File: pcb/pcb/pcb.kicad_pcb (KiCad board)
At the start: 2 copper layers, 66 x 44.5 mm, 20 parts, among them J1 UART, J2 Barrel_Jack, J3 Stepper, SW1 RESET, SW2 FLASH, U1 ESP32-WROOM-32, U2 TSR_1-2433

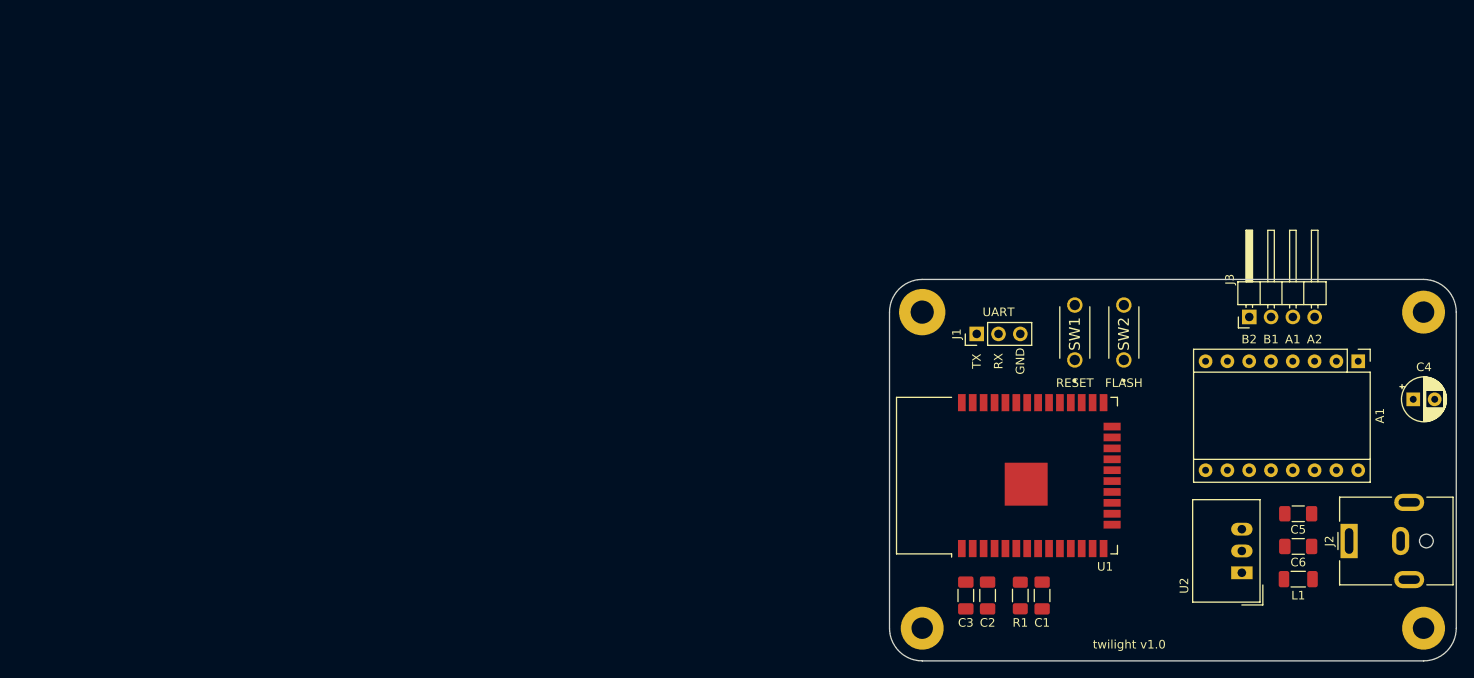
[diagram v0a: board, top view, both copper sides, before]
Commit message: route traces
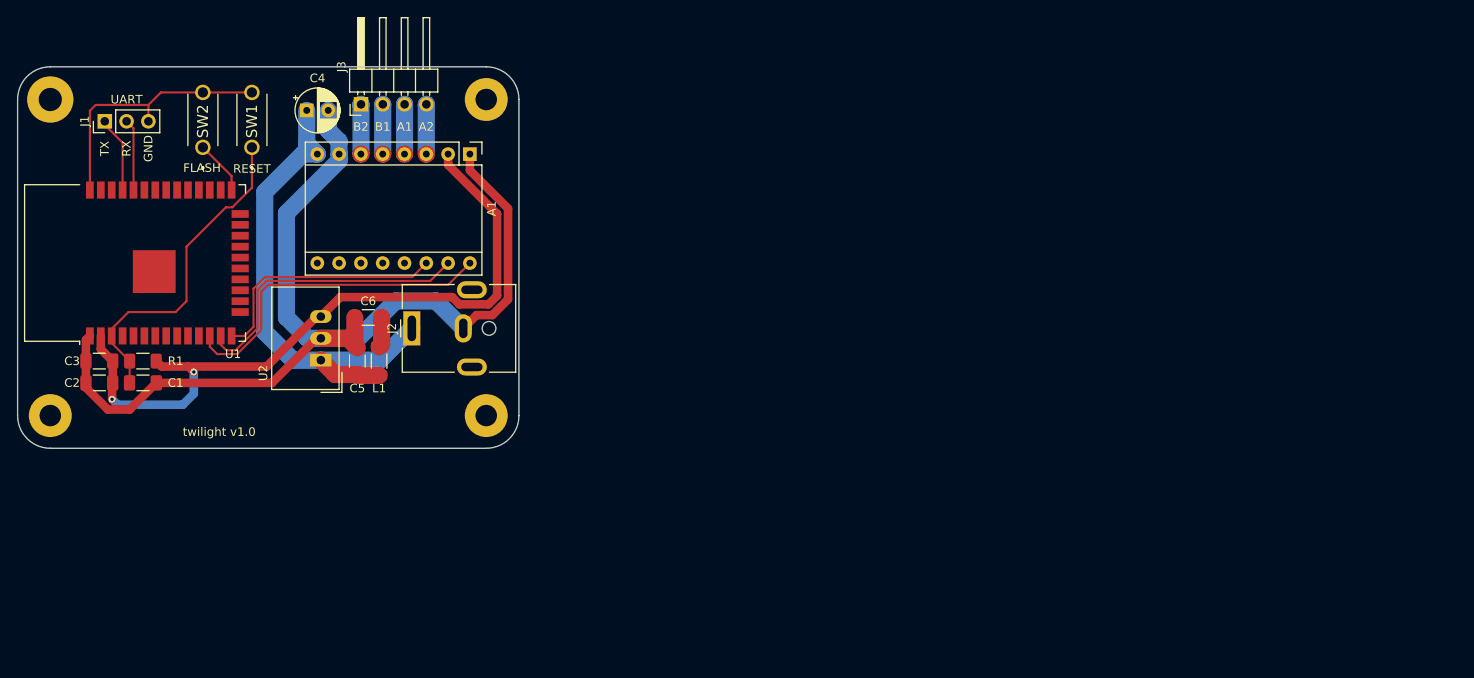
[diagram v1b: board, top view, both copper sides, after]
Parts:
- moved C4 133.3 mm to (111.2, 48.9)
- moved H2 112.0 mm to (132.1, 47.6)
- moved H4 112.0 mm to (132.1, 84.4)
- moved J2 112.0 mm to (123.4, 74.3)
- moved C6 111.6 mm to (118.3, 73.0)
- moved C5 111.1 mm to (117.1, 78.1), turned to 90 degrees
- moved SW2 110.1 mm to (99.1, 53.2)
- moved U2 110.1 mm to (112.8, 78.0)
- moved L1 110.1 mm to (119.6, 78.1), turned to 90 degrees
- moved C1 107.7 mm to (92.1, 80.6), turned to 0 degrees
- moved J3 106.4 mm to (117.5, 48.2)
- moved C2 106.4 mm to (87.0, 80.6), turned to 180 degrees
- moved A1 106.3 mm to (130.2, 54.0)
- moved R1 105.8 mm to (92.1, 78.1), turned to 180 degrees
- moved C3 104.6 mm to (87.0, 78.1), turned to 180 degrees
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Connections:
- net Net-(C1-Pad1) renamed /EN
- U1 pad 12: unconnected-(U1-Pad12) -> /DIR
- U1 pad 13: unconnected-(U1-Pad13) -> /STEP
- U1 pad 14: unconnected-(U1-Pad14) -> /SLP
- U1 pad 6: /DIR -> unconnected-(U1-Pad6)
- U1 pad 7: /SLP -> unconnected-(U1-Pad7)
- U1 pad 9: /STEP -> unconnected-(U1-Pad9)
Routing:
- net GND: track 0.00 -> 154.2 mm
- net +3V3: track 0.00 -> 84.3 mm, vias 0 -> 2
- net +12V: track 0.00 -> 57.4 mm
- net /DIR: track 0.00 -> 38.9 mm
- net /EN: track 0.00 -> 38.7 mm
- net /STEP: track 0.00 -> 34.6 mm
- net /SLP: track 0.00 -> 28.8 mm
- net /TX: track 0.00 -> 8.87 mm
- net /RX: track 0.00 -> 8.34 mm
- net IO0: track 0.00 -> 6.36 mm
- net /B2: track 0.00 -> 5.81 mm
- net /B1: track 0.00 -> 5.81 mm
- net /A2: track 0.00 -> 5.81 mm
- net /A1: track 0.00 -> 5.81 mm
- net Net-(C6-Pad1): track 0.00 -> 3.54 mm
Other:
- board size 66 x 44.5 mm -> 58.4 x 44.4 mm
